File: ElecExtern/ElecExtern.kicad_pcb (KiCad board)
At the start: 2 copper layers, 91.4 x 78.7 mm, 26 parts, among them J1 Conn_01x02, J2 Conn_01x04, J3 Conn_01x02, J4 Conn_01x02, J5 Conn_01x02, Q1 Q_NMOS_DGS, Q2 Q_NMOS_DGS, U1 R-78C3.3-1.0, U2 PMOS, U3 Xbee802.15.4, U4 SD_card

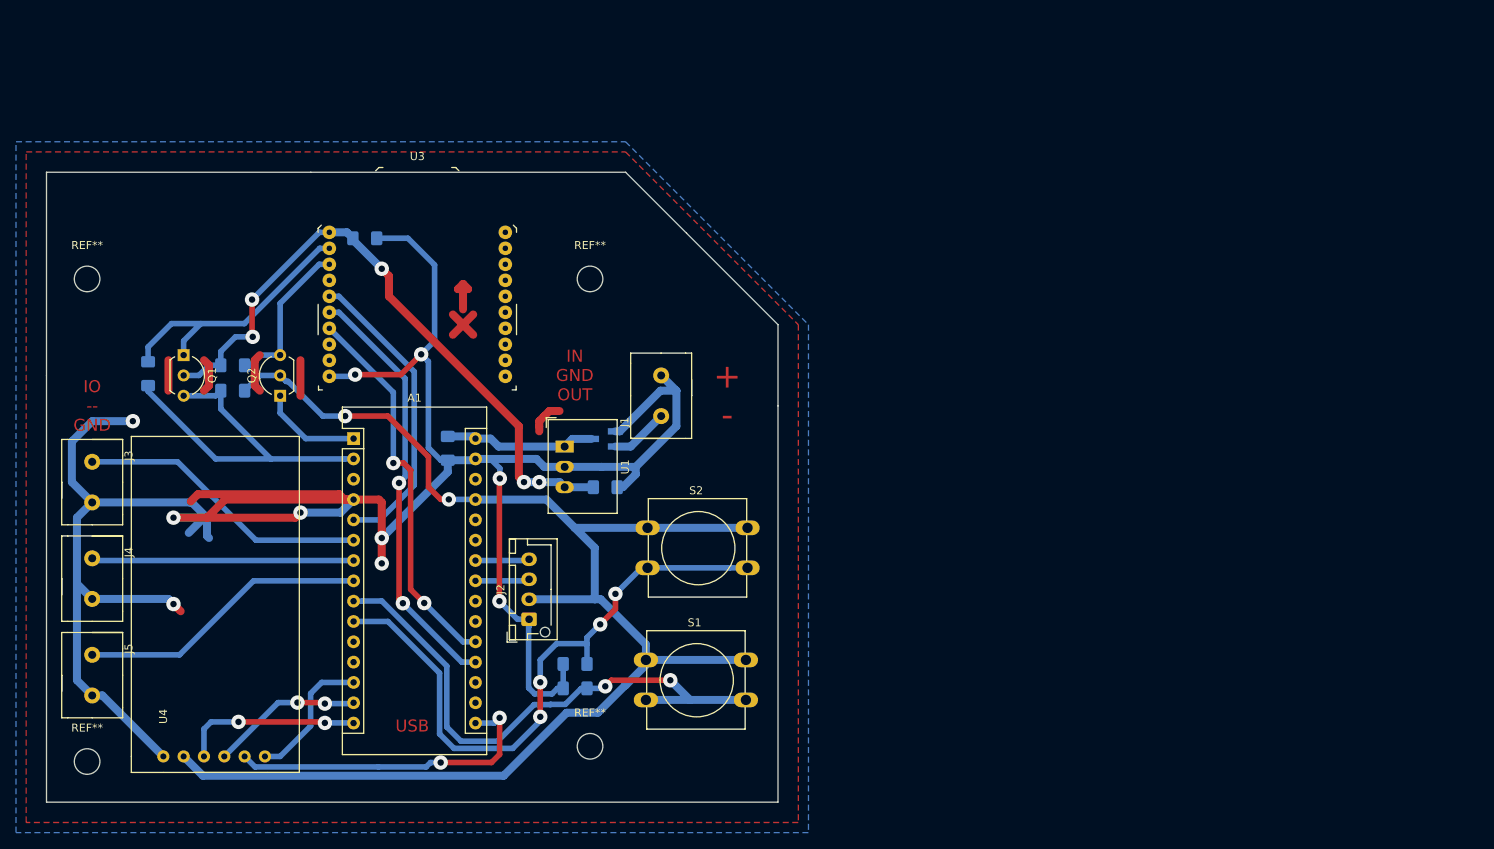
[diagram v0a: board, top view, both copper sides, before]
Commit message: Grosse mise à jour
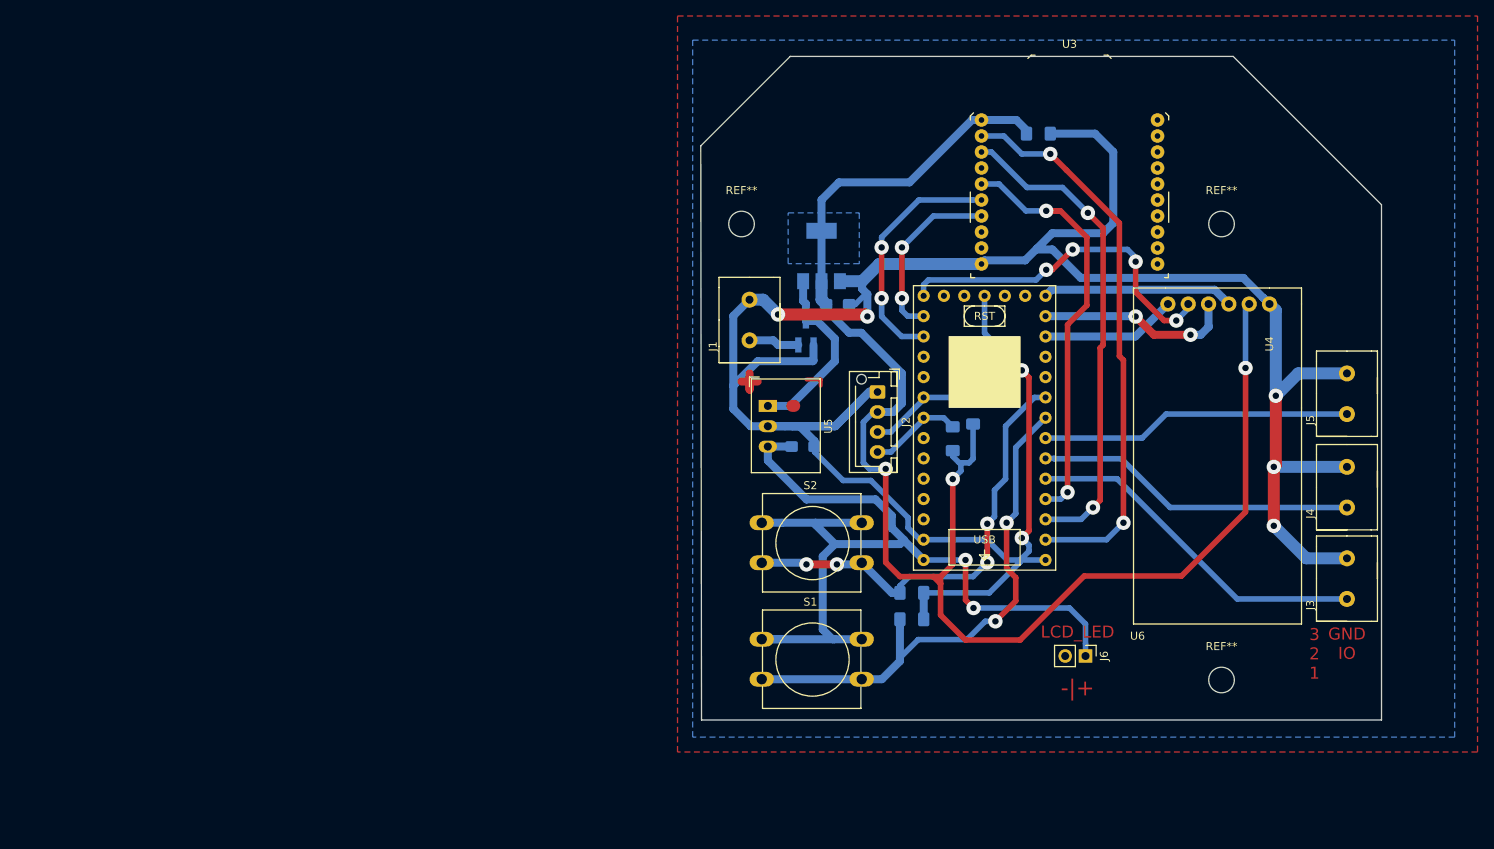
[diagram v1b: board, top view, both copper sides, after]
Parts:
- removed A1: Arduino_Nano_v3.x, Module:Arduino_Nano
- removed JP1: SolderJumper_2_Open, Resistor_SMD:R_1206_3216Metric_Pad1.42x1.75mm_HandSolder
- removed Q1, Q2: Q_NMOS_DGS, Package_TO_SOT_THT:TO-92L_Inline_Wide
- removed the REF** at (76.2, 123.2)
- removed the REF** at (139.1, 121.3)
- removed the REF** at (139.1, 62.9)
- removed the REF** at (76.2, 62.9)
- added J6: Conn_01x02, Connector_PinHeader_2.54mm:PinHeader_1x02_P2.54mm_Vertical, F.Cu at (201.0, 110.0)
- added REF**: MountingHole_3.2mm_M3, MountingHole:MountingHole_3.2mm_M3, F.Cu at (158.0, 56.0)
- added REF**: MountingHole_3.2mm_M3, MountingHole:MountingHole_3.2mm_M3, F.Cu at (218.0, 113.0)
- added REF**: MountingHole_3.2mm_M3, MountingHole:MountingHole_3.2mm_M3, F.Cu at (218.0, 56.0)
- added U5: R-78C5.0-1.0, Converter_DCDC:Converter_DCDC_RECOM_R-78E-0.5_THT, F.Cu at (161.3, 78.7)
- added U6: TEENSY3.2, RTS:TEENSY3.2_RTS, F.Cu at (196.0, 98.0)
- C2: value C -> 10uF_tantalum_AMS1117; footprint Capacitor_SMD:C_1206_3216Metric_Pad1.42x1.75mm_HandSolder -> Capacitor_Tantalum_SMD:CP_EIA-3216-18_Kemet-A_Pad1.58x1.35mm_HandSolder
- C3: value 10uF -> 10uf MLCC; footprint Capacitor_SMD:C_1206_3216Metric_Pad1.42x1.75mm_HandSolder -> Capacitor_Tantalum_SMD:CP_EIA-3216-18_Kemet-A_Pad1.58x1.35mm_HandSolder
- R3, R4: value 1kR pull-up -> R
- U1: value R-78C3.3-1.0 -> AMS1117-3.3; footprint Converter_DCDC:Converter_DCDC_RECOM_R-78E-0.5_THT -> Package_TO_SOT_SMD:SOT-223-3_TabPin2; moved to B.Cu
- moved J5 160.7 mm to (233.7, 77.2), turned to 90 degrees
- moved J3 157.3 mm to (233.7, 100.3), turned to 90 degrees
- moved J4 157.3 mm to (233.7, 88.9), turned to 90 degrees
- moved U4 149.4 mm to (224.0, 66.0), turned to 270 degrees
- moved R3 92.6 mm to (186.9, 79.5), turned to 270 degrees
- moved R4 90.5 mm to (184.4, 82.8), turned to 270 degrees
- moved C1 85.2 mm to (195.1, 44.7)
- moved U3 82.7 mm to (199.0, 52.0)
- moved J2 52.0 mm to (175.0, 77.0), turned to 270 degrees
- moved C2 51.9 mm to (170.0, 66.0), turned to 0 degrees
- moved R2 43.0 mm to (179.3, 102.1), turned to 180 degrees
- moved R1 43.0 mm to (179.3, 105.4), turned to 180 degrees
- moved U1 40.0 mm to (168.0, 60.0), turned to 90 degrees
- moved U2 28.6 mm to (166.1, 69.6), turned to 90 degrees
- moved C3 25.2 mm to (165.7, 83.8)
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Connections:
- C2 pad 1: +12V -> +3V3
- C3 pad 1: +3V3 -> +5V
- J2 pad 2: +5V -> +3V3
- R3 pad 1: +5V -> /SDA
- R3 pad 2: /RX_Duino -> +3V3
- R4 pad 1: +3V3 -> /SCL
- R4 pad 2: /DIN -> +3V3
- U1 pad 1: +12V -> GND
- U1 pad 2: GND -> +3V3
- U1 pad 3: +3V3 -> +12V
- U4 pad 2: +5V -> +3V3
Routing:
- net +3V3: track 81.0 -> 195.7 mm, vias 5 -> 3
- net +5V: track 180.1 -> 114.1 mm
- net /RX_Duino: track 45.9 -> 0.00 mm
- net /DIN: track 19.6 -> 61.1 mm, vias 0 -> 2
- net /DOUT: track 34.4 -> 70.0 mm, vias 0 -> 2
- net (no net): track 35.3 -> 7.37 mm
- net /PWM1_XBEE: track 48.4 -> 22.5 mm
- net /PWM0_XBEE: track 53.6 -> 30.6 mm
- net /Bouton2_IN: track 78.2 -> 56.5 mm
- net /Xbee-reset: track 38.1 -> 52.7 mm, vias 0 -> 2
- net /TX_Duino: track 12.7 -> 0.00 mm
- net GND: track 322.5 -> 333.2 mm, vias 10 -> 7
- net /IO2: track 32.8 -> 40.2 mm
- net /SDA: track 6.78 -> 14.0 mm
- net /IO1: track 36.7 -> 43.9 mm
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- added copper zone on B.Cu, net +3V3
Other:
- board size 91.4 x 78.7 mm -> 85.1 x 82.9 mm
- board text added: "-|+"
- board text added: "3 2 1"
- board text added: "GND IO"
- board text added: "LCD_LED"
- board text removed: "+ -"
- board text removed: "IN GND OUT"
- board text removed: "IO -- GND"
- board text removed: "USB"
